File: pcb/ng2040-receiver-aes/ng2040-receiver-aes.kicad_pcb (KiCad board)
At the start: 2 copper layers, 32 x 33.5 mm, 20 parts, among them J1 DB15_F, SW1 OPTS, U1 RP2040-Zero, U2 NRF24L01_Breakout

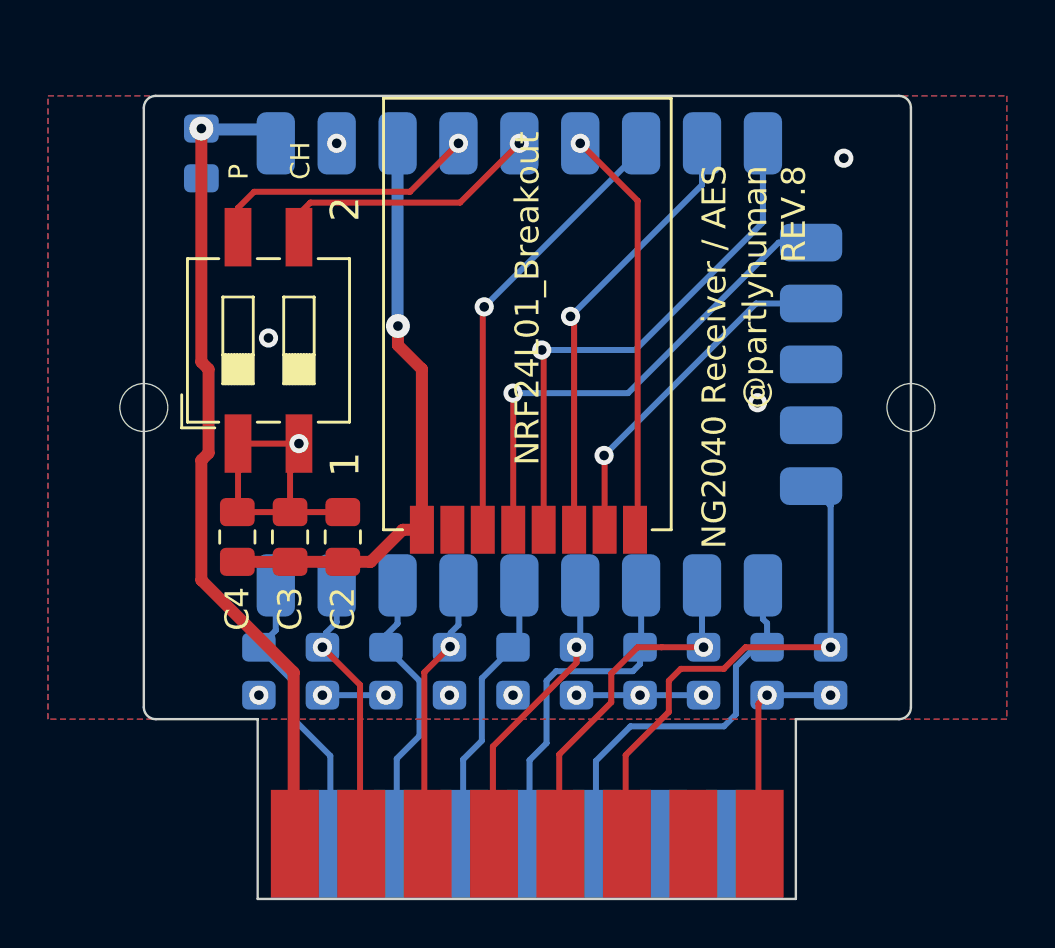
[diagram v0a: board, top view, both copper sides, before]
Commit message: AES shave down
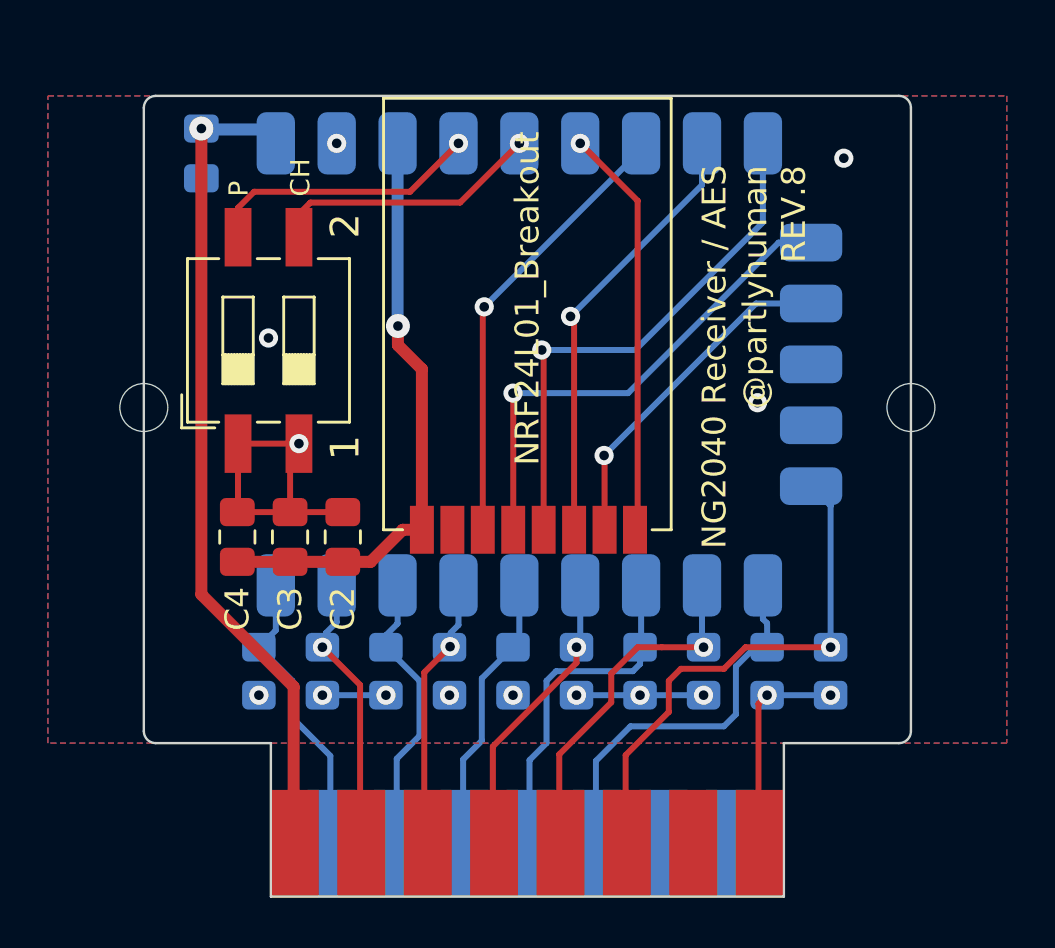
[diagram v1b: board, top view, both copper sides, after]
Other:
- board size 32 x 33.5 mm -> 32 x 33.4 mm
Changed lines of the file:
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@@
 	(generator_version "9.0")
 	(general
-		(thickness 1.6)
+		(thickness 1.2)
 		(legacy_teardrops no)
 	)
@@
 			(layer "dielectric 1"
 				(type "core")
-				(thickness 1.51)
+				(thickness 1.11)
 				(material "FR4")
 				(epsilon_r 4.5)
@@
 	)
 	(gr_line
-		(start 84 82.5)
+		(start 84 83.5)
 		(end 84 69)
 		(stroke
@@
 	)
 	(gr_line
-		(start 116 82.5)
+		(start 116 83.5)
 		(end 116 69)
 		(stroke
@@
 	)
 	(gr_arc
-		(start 84.5 83)
-		(mid 84.146447 82.853553)
-		(end 84 82.5)
+		(start 115.5 57)
+		(mid 115.853553 57.146447)
+		(end 116 57.5)
 		(stroke
 			(width 0.1)
@@
 	)
 	(gr_arc
-		(start 116 82.5)
-		(mid 115.853553 82.853553)
-		(end 115.5 83)
+		(start 116 83.5)
+		(mid 115.853553 83.853553)
+		(end 115.5 84)
 		(stroke
 			(width 0.1)
@@
 		(layer "Edge.Cuts")
 	)
-	(gr_arc
-		(start 115.5 57)
-		(mid 115.853553 57.146447)
-		(end 116 57.5)
+	(gr_line
+		(start 115.5 84)
+		(end 110.7 84)
 		(stroke
 			(width 0.1)
@@
 	)
 	(gr_line
-		(start 88.75 83)
-		(end 88.75 90.5)
+		(start 84.5 84)
+		(end 89.3 84)
 		(stroke
 			(width 0.1)
@@
 	)
 	(gr_line
-		(start 84 69)
-		(end 84 57.5)
+		(start 89.3 84)
+		(end 89.3 90.4)
 		(stroke
 			(width 0.1)
@@
 	)
 	(gr_line
-		(start 88.75 90.5)
-		(end 111.2 90.5)
+		(start 84 69)
+		(end 84 57.5)
 		(stroke
 			(width 0.1)
@@
 	)
 	(gr_line
-		(start 111.2 90.5)
-		(end 111.2 83)
+		(start 89.3 90.4)
+		(end 110.7 90.4)
 		(stroke
 			(width 0.1)
@@
 	)
 	(gr_line
-		(start 115.5 83)
-		(end 111.2 83)
+		(start 110.7 90.4)
+		(end 110.7 84)
 		(stroke
 			(width 0.1)
@@
 		(layer "Edge.Cuts")
 	)
-	(gr_line
-		(start 84.5 83)
-		(end 88.75 83)
+	(gr_arc
+		(start 84.5 84)
+		(mid 84.146447 83.853553)
+		(end 84 83.5)
 		(stroke
 			(width 0.1)
@@
 	)
 	(gr_text "2"
-		(at 93.1 61.2 90)
+		(at 93.1 61.9 90)
 		(layer "F.SilkS")
 		(effects
@@
 	)
 	(gr_text "1"
-		(at 93.1 72.9 90)
+		(at 93.1 72.2 90)
 		(layer "F.SilkS")
 		(effects
@@
 	)
 	(gr_text "P\n\nCH"
-		(at 91 60.5 90)
+		(at 91 61.2 90)
 		(layer "F.SilkS")
 		(effects
@@
 	(segment
 		(start 86.4 58.3625)
-		(end 86.4 68.1)
-		(width 0.5)
-		(layer "F.Cu")
-		(net 2)
-	)
-	(segment
-		(start 86.4 68.1)
-		(end 86.7 68.4)
-		(width 0.5)
-		(layer "F.Cu")
-		(net 2)
-	)
-	(segment
-		(start 86.4 77.2)
-		(end 90.25 81.05)
-		(width 0.5)
-		(layer "F.Cu")
-		(net 2)
-	)
-	(segment
-		(start 86.4 72.2)
-		(end 86.4 77.2)
-		(width 0.5)
-		(layer "F.Cu")
-		(net 2)
-	)
-	(segment
-		(start 86.7 71.9)
-		(end 86.4 72.2)
+		(end 86.4 77.8)
 		(width 0.5)
 		(layer "F.Cu")
@@
 	)
 	(segment
-		(start 86.7 68.4)
-		(end 86.7 71.9)
+		(start 86.4 77.8)
+		(end 90.25 81.65)
 		(width 0.5)
 		(layer "F.Cu")
@@
 	)
 	(segment
-		(start 90.25 81.05)
+		(start 90.25 81.65)
 		(end 90.25 88)
 		(width 0.5)
@@
 		(polygon
 			(pts
-				(xy 120 83) (xy 80 83) (xy 80 57) (xy 120 57)
+				(xy 120 84) (xy 80 84) (xy 80 57) (xy 120 57)
 			)
 		)
